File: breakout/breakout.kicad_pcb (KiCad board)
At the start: 2 copper layers, 50 x 50 mm, 23 parts, among them P1 CONN_01X07, P4 CONN_01X04, P5 CONN_01X07, P6 CONN_01X04

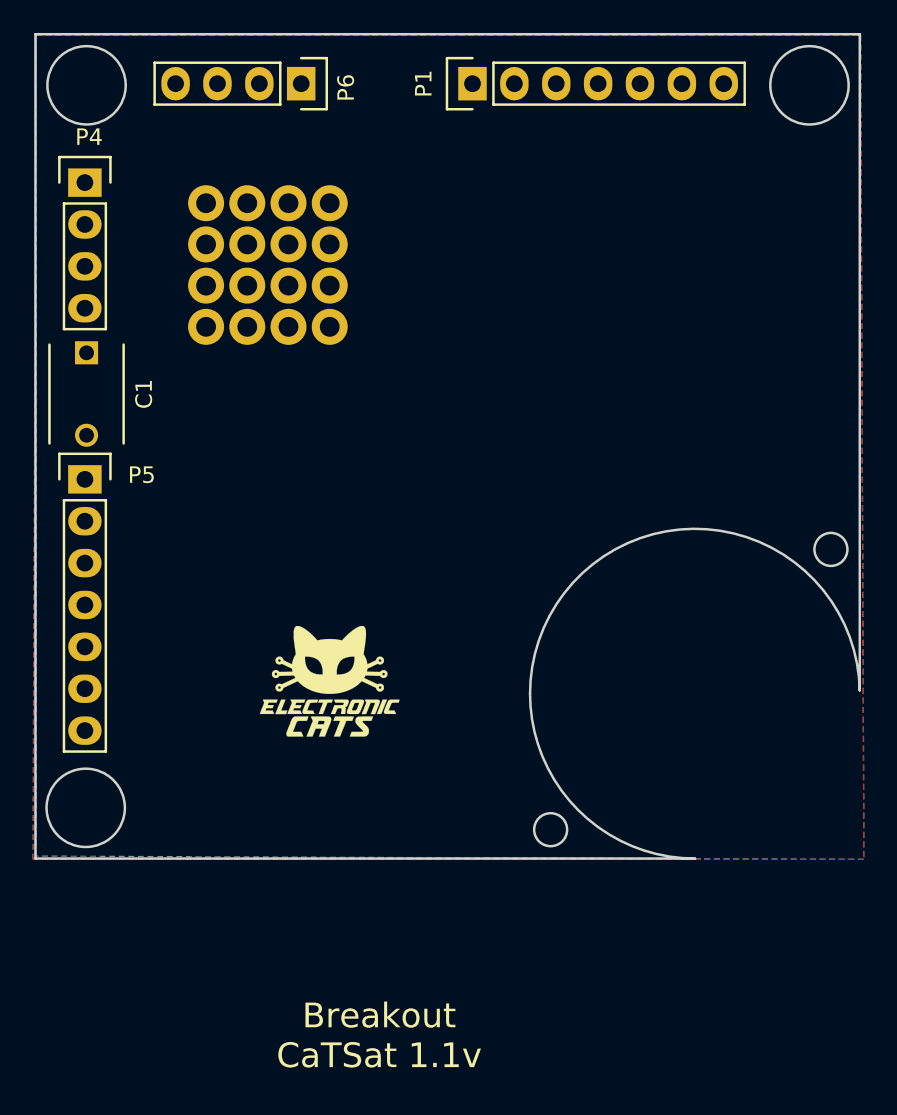
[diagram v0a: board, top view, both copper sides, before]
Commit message: Update payload
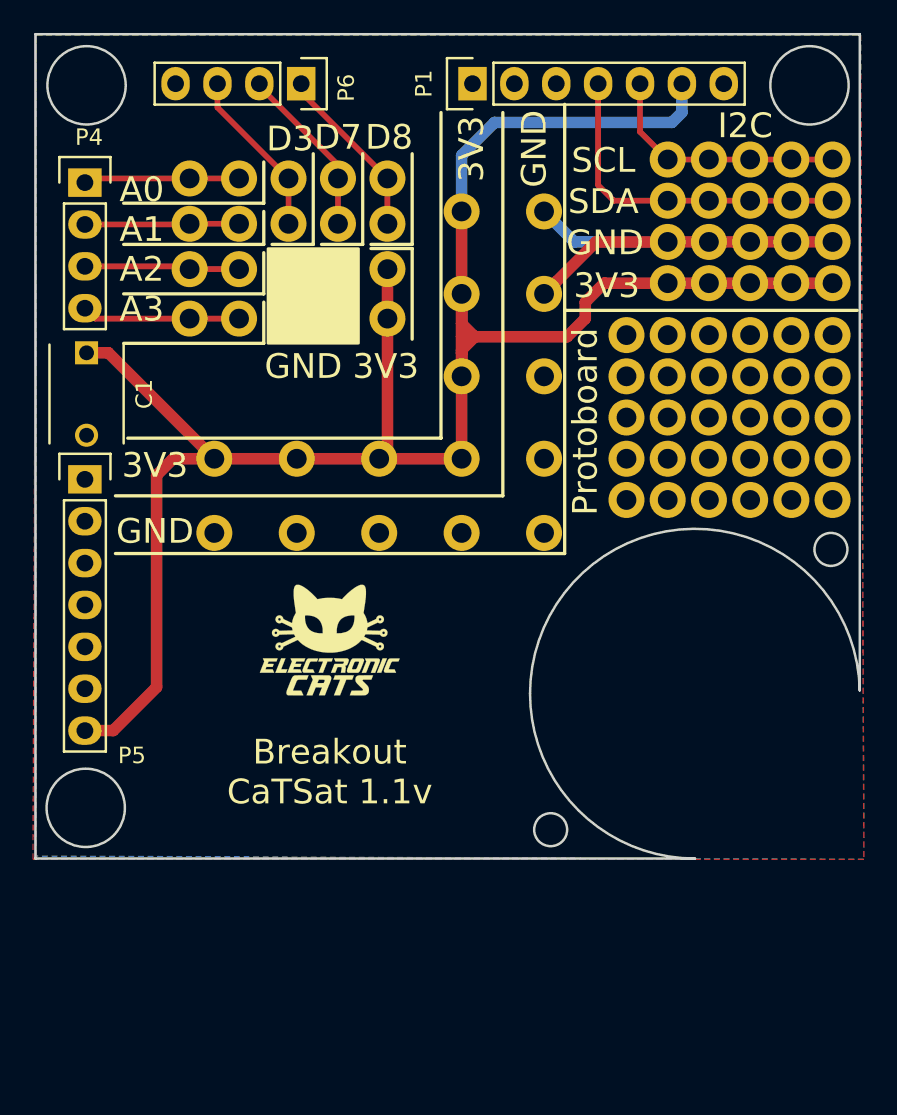
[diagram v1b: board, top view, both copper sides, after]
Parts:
- removed the REF** at (124.5, 92.0)
- added J1: D7, CatSat:Pin, F.Cu at (126.5, 91.5)
- added J10: D7, CatSat:Pin, F.Cu at (123.5, 91.5)
- added J11: D7, CatSat:Pin, F.Cu at (132.5, 83.0)
- added J12: D7, CatSat:Pin, F.Cu at (132.5, 85.8)
- added J13: D7, CatSat:Pin, F.Cu at (152.5, 89.3)
- added J13: D7, CatSat:Pin, F.Cu at (155.0, 89.3)
- added J13: D7, CatSat:Pin, F.Cu at (157.5, 89.3)
- added J13: D7, CatSat:Pin, F.Cu at (160.0, 89.3)
- added J13: D7, CatSat:Pin, F.Cu at (162.5, 89.3)
- added J14: D7, CatSat:Pin, F.Cu at (140.0, 85.0)
- added J14: D7, CatSat:Pin, F.Cu at (140.0, 90.0)
- added J14: D7, CatSat:Pin, F.Cu at (140.0, 95.0)
- added J14: D7, CatSat:Pin, F.Cu at (140.0, 100.0)
- added J14: D7, CatSat:Pin, F.Cu at (135.0, 100.0)
- added J14: D7, CatSat:Pin, F.Cu at (130.0, 100.0)
- added J14: D7, CatSat:Pin, F.Cu at (125.0, 100.0)
- added J16: D7, CatSat:Pin, F.Cu at (135.5, 91.5)
- added J17: D7, CatSat:Pin, F.Cu at (135.5, 88.5)
- added J18: D7, CatSat:Pin, F.Cu at (157.5, 81.8)
- added J19: D7, CatSat:Pin, F.Cu at (155.0, 81.8)
- added J2: D7, CatSat:Pin, F.Cu at (129.5, 83.0)
- added J20: D7, CatSat:Pin, F.Cu at (152.5, 81.8)
- added J21: D7, CatSat:Pin, F.Cu at (162.5, 81.8)
- added J22: D7, CatSat:Pin, F.Cu at (160.0, 81.8)
- added J23: D7, CatSat:Pin, F.Cu at (135.5, 85.8)
- added J24: D7, CatSat:Pin, F.Cu at (135.5, 83.0)
- added J26: D7, CatSat:Pin, F.Cu at (129.5, 88.5)
- added J27: D7, CatSat:Pin, F.Cu at (132.5, 88.5)
- added J27: D7, CatSat:Pin, F.Cu at (132.5, 91.5)
- added J27: D7, CatSat:Pin, F.Cu at (129.5, 91.5)
- added J28: D7, CatSat:Pin, F.Cu at (152.5, 86.8)
- added J28: D7, CatSat:Pin, F.Cu at (155.0, 86.8)
- added J28: D7, CatSat:Pin, F.Cu at (157.5, 86.8)
- added J28: D7, CatSat:Pin, F.Cu at (160.0, 86.8)
- added J28: D7, CatSat:Pin, F.Cu at (162.5, 86.8)
- added J29: D7, CatSat:Pin, F.Cu at (145.0, 85.0)
- added J29: D7, CatSat:Pin, F.Cu at (145.0, 90.0)
- added J29: D7, CatSat:Pin, F.Cu at (145.0, 95.0)
- added J29: D7, CatSat:Pin, F.Cu at (145.0, 100.0)
- added J29: D7, CatSat:Pin, F.Cu at (145.0, 104.5)
- added J29: D7, CatSat:Pin, F.Cu at (140.0, 104.5)
- added J29: D7, CatSat:Pin, F.Cu at (135.0, 104.5)
- added J29: D7, CatSat:Pin, F.Cu at (130.0, 104.5)
- added J29: D7, CatSat:Pin, F.Cu at (125.0, 104.5)
- added J3: D7, CatSat:Pin, F.Cu at (129.5, 85.8)
- added J30: D7, CatSat:Pin, F.Cu at (152.5, 84.3)
- added J31: D7, CatSat:Pin, F.Cu at (160.0, 84.3)
- added J32: D7, CatSat:Pin, F.Cu at (162.5, 84.3)
- added J33: D7, CatSat:Pin, F.Cu at (157.5, 84.3)
- added J34: D7, CatSat:Pin, F.Cu at (155.0, 84.3)
- added J4: D7, CatSat:Pin, F.Cu at (126.5, 85.8)
- added J5: D7, CatSat:Pin, F.Cu at (126.5, 88.5)
- added J6: D7, CatSat:Pin, F.Cu at (123.5, 85.8)
- added J7: D7, CatSat:Pin, F.Cu at (123.5, 88.5)
- added J8: D7, CatSat:Pin, F.Cu at (123.5, 83.0)
- added J9: D7, CatSat:Pin, F.Cu at (126.5, 83.0)
- added REF**: Pin, CatSat:Pin, F.Cu at (150.0, 92.5)
- added REF**: Pin, CatSat:Pin, F.Cu at (162.5, 102.5)
- added REF**: Pin, CatSat:Pin, F.Cu at (160.0, 102.5)
- added REF**: Pin, CatSat:Pin, F.Cu at (157.5, 102.5)
- added REF**: Pin, CatSat:Pin, F.Cu at (155.0, 102.5)
- added REF**: Pin, CatSat:Pin, F.Cu at (160.0, 100.0)
- added REF**: Pin, CatSat:Pin, F.Cu at (162.5, 100.0)
- added REF**: Pin, CatSat:Pin, F.Cu at (152.5, 92.5)
- added REF**: Pin, CatSat:Pin, F.Cu at (155.0, 92.5)
- added REF**: Pin, CatSat:Pin, F.Cu at (152.5, 95.0)
- added REF**: Pin, CatSat:Pin, F.Cu at (152.5, 97.5)
- added REF**: Pin, CatSat:Pin, F.Cu at (152.5, 100.0)
- added REF**: Pin, CatSat:Pin, F.Cu at (152.5, 102.5)
- added REF**: Pin, CatSat:Pin, F.Cu at (155.0, 100.0)
- added REF**: Pin, CatSat:Pin, F.Cu at (157.5, 100.0)
- P1, P5: value CONN_01X07 -> Conn_01x07_Male
- P4, P6: value CONN_01X04 -> Conn_01x04_Male
- moved REF** 32.3 mm to (162.5, 95.0)
- moved REF** 32.3 mm to (162.5, 97.5)
- moved REF** 32.3 mm to (160.0, 97.5)
- moved REF** 32.3 mm to (157.5, 97.5)
- moved REF** 32.3 mm to (155.0, 97.5)
- moved REF** 32.3 mm to (160.0, 95.0)
- moved REF** 32.3 mm to (157.5, 95.0)
- moved REF** 32.3 mm to (155.0, 95.0)
- moved REF** 30.5 mm to (162.5, 92.5)
- moved REF** 30.5 mm to (160.0, 92.5)
- moved REF** 30.5 mm to (157.5, 92.5)
- moved REF** 28.6 mm to (150.0, 102.5), turned to 90 degrees
- moved REF** 25.3 mm to (150.0, 100.0), turned to 90 degrees
- moved REF** 22.0 mm to (150.0, 97.5), turned to 90 degrees
- moved REF** 18.8 mm to (150.0, 95.0), turned to 90 degrees
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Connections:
- P1 pad 1: GND -> /DHT/D6
- P1 pad 2: +BATT -> /S_TX
- P1 pad 3: /SCL -> /S_RX
- P1 pad 5: /S_RX -> /SCL
- P1 pad 6: /S_TX -> +BATT
- P1 pad 7: /DHT/D6 -> GND
- P4 pad 1: /A3 -> /A0
- P4 pad 2: /A2 -> /A1
- P4 pad 3: /A1 -> /A2
- P4 pad 4: /A0 -> /A3
- P5 pad 1: +BATT -> /RST
- P5 pad 2: GND -> /NSS
- P5 pad 3: /SCK -> /MOSI
- P5 pad 5: /MOSI -> /SCK
- P5 pad 6: /NSS -> GND
- P5 pad 7: /RST -> +BATT
- P6 pad 1: /INT0 -> /D8
- P6 pad 2: /INT1 -> /D7
- P6 pad 3: /D7 -> /INT1
- P6 pad 4: /D8 -> /INT0
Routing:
- net +BATT: track 0.00 -> 135.8 mm
- net GND: track 0.00 -> 28.1 mm
- net /SDA: track 0.00 -> 20.8 mm
- net /SCL: track 0.00 -> 15.3 mm
- net /D8: track 0.00 -> 10.7 mm
- net /D7: track 0.00 -> 10.5 mm
- net /INT1: track 0.00 -> 10.3 mm
- net /A0: track 0.00 -> 9.95 mm
- net /A3: track 0.00 -> 9.61 mm
- net /A2: track 0.00 -> 9.42 mm
- net /A1: track 0.00 -> 9.37 mm
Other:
- net class Default: trace_width 0.3 -> 0.35
- net class vcc: trace_width 0.5 -> 0.7
- board text added: "3V3"
- board text added: "A0 A1 A2 A3"
- board text added: "D3"
- board text added: "D7"
- board text added: "D8"
- board text added: "GND"
- board text added: "I2C"
- board text added: "Protoboard"
- board text added: "SCL"
- board text added: "SDA"
- board text removed: "D6 DHT"
- board text removed: "SCL SDA"
- board text removed: "S_RX S_TX"
